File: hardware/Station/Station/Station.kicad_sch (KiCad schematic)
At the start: 7 parts, among them J1 Conn_01x04, J2 Conn_01x04, J3 Conn_01x04, J4 Conn_01x04, J5 Conn_01x04, J6 Conn_01x03

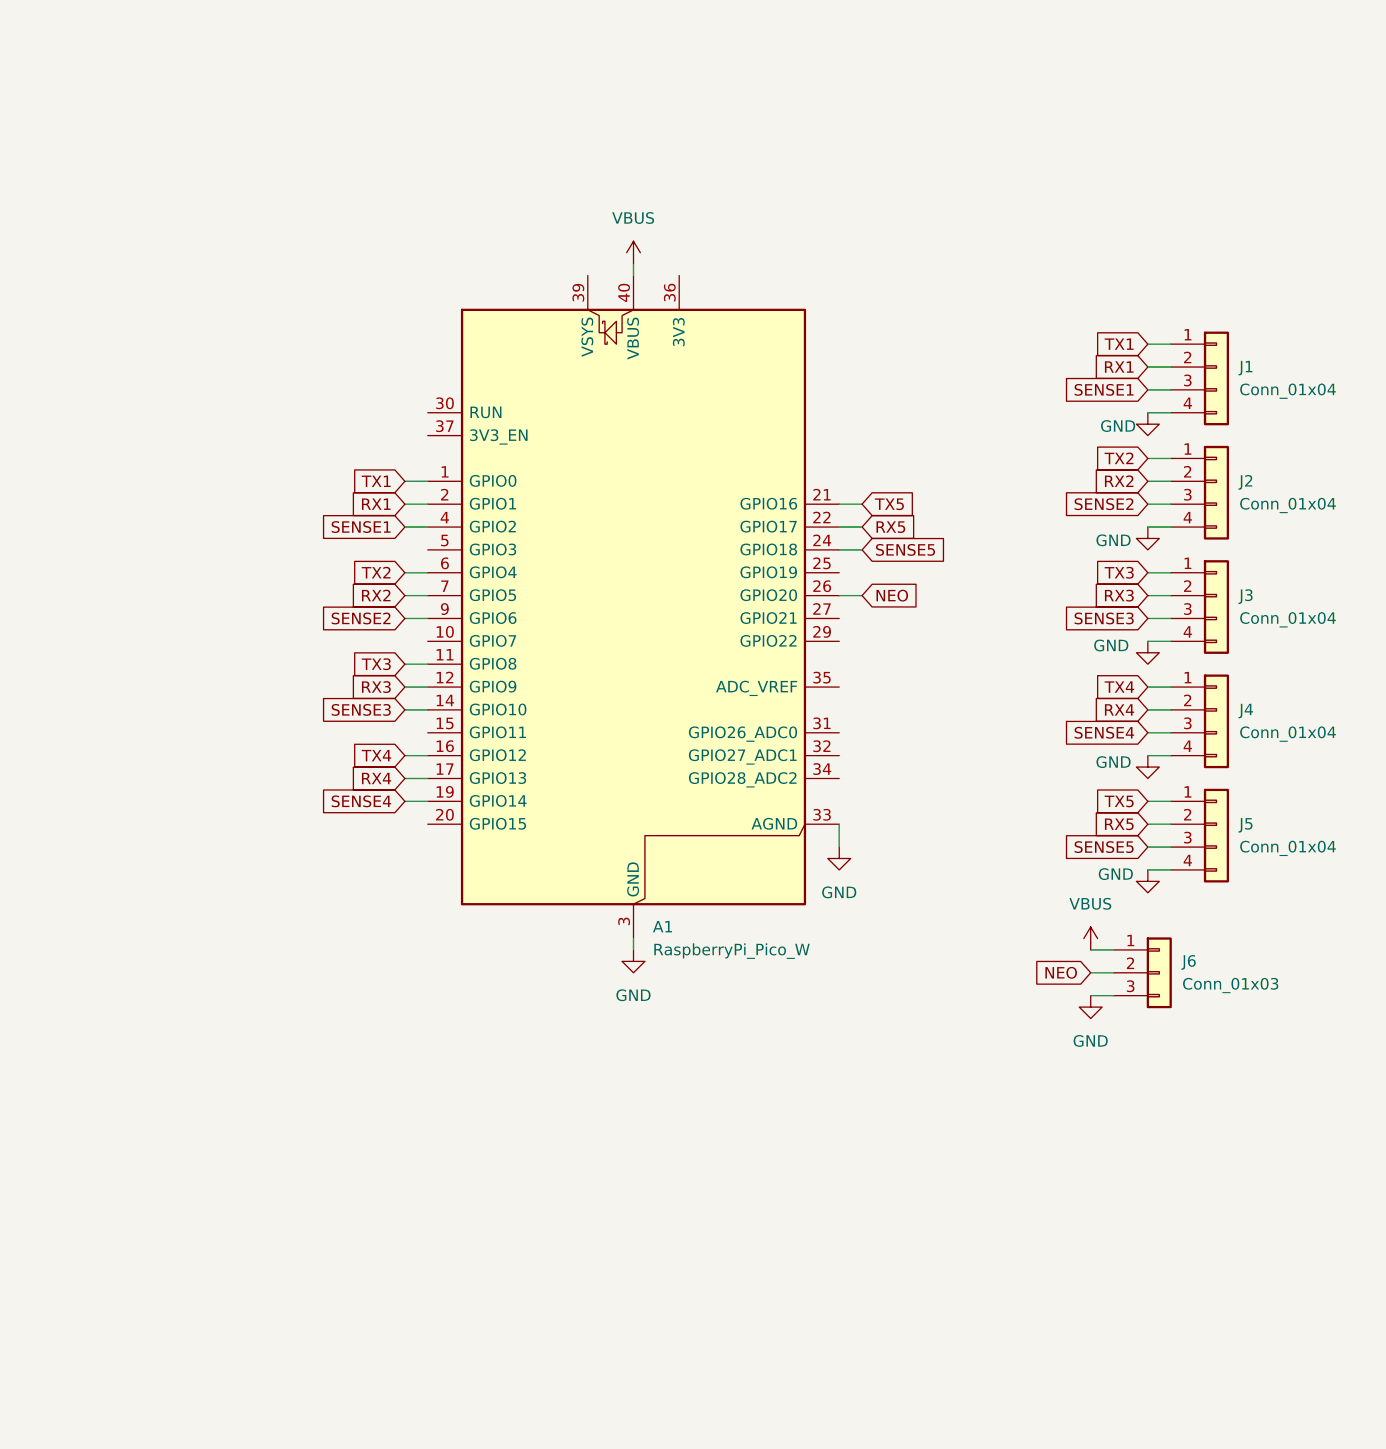
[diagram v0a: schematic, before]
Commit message: V1.0 firmware release
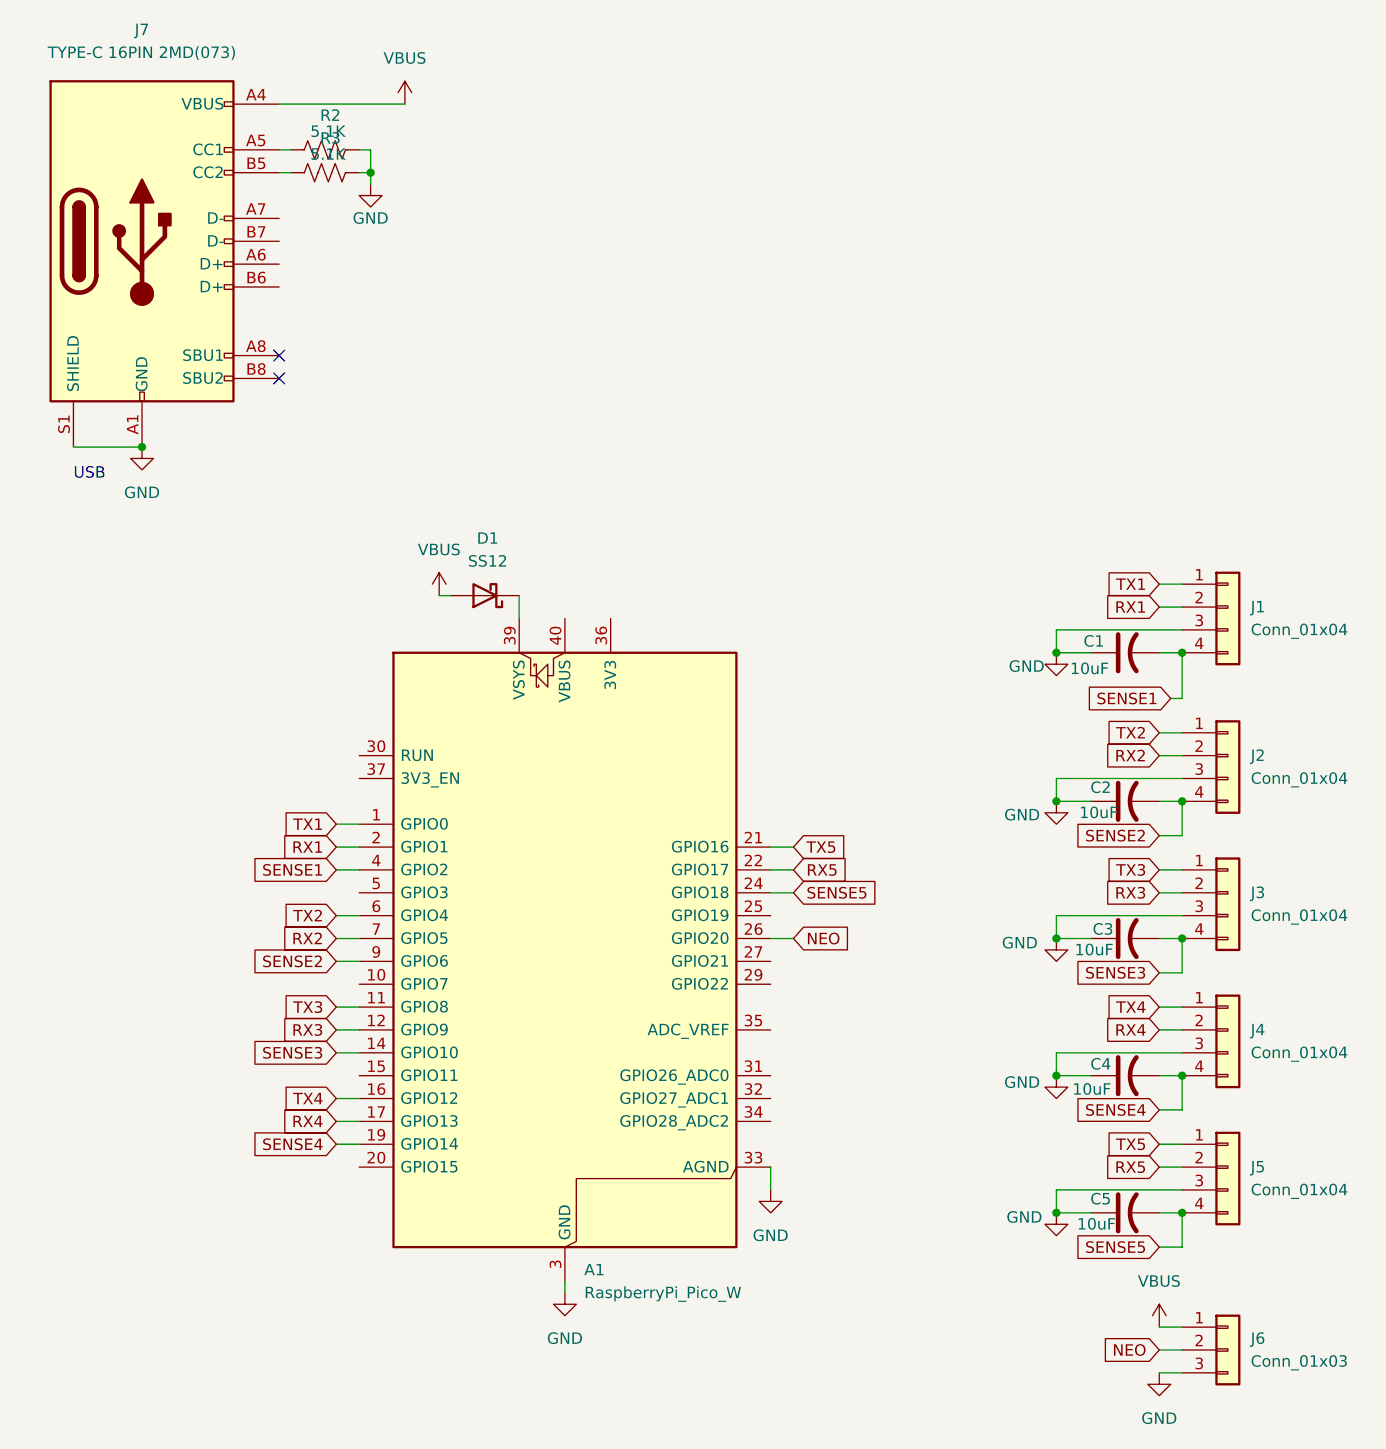
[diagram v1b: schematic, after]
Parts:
- added C1, C2, C3, C4, C5: 10uF, Capacitor_SMD:C_0603_1608Metric_Pad1.08x0.95mm_HandSolder, symbol Device:C_US
- added D1: SS12, Diode_SMD:D_SMA, symbol Diode:SS12
- added J7: TYPE-C 16PIN 2MD(073), Connector_USB:USB_C_Receptacle_GCT_USB4105-xx-A_16P_TopMnt_Horizontal, symbol Connector:USB_C_Receptacle_USB2.0
- added R2, R3: 5.1K, Resistor_SMD:R_0603_1608Metric, symbol Device:R_US
- J1, J2, J3, J4, J5: footprint Connector_PinHeader_1.27mm:PinHeader_1x04_P1.27mm_Vertical -> Connector_PinHeader_2.54mm:PinHeader_1x04_P2.54mm_Vertical
- J6: footprint (none) -> Connector_PinHeader_2.54mm:PinHeader_1x03_P2.54mm_Vertical
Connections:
- net GND: now also J1.3 (Pin_3), J2.3 (Pin_3), J3.3 (Pin_3), J4.3 (Pin_3), J5.3 (Pin_3), C1.1, C2.1, C3.1, C4.1, C5.1, J7.A1 (GND), J7.A12 (GND), J7.B1 (GND), J7.B12 (GND), J7.S1 (SHIELD), R2.2, R3.2; no longer J1.4 (Pin_4), J2.4 (Pin_4), J3.4 (Pin_4), J4.4 (Pin_4), J5.4 (Pin_4)
- net SENSE1: now also J1.4 (Pin_4), C1.2; no longer J1.3 (Pin_3)
- net SENSE2: now also J2.4 (Pin_4), C2.2; no longer J2.3 (Pin_3)
- net SENSE3: now also J3.4 (Pin_4), C3.2; no longer J3.3 (Pin_3)
- net SENSE4: now also J4.4 (Pin_4), C4.2; no longer J4.3 (Pin_3)
- net SENSE5: now also J5.4 (Pin_4), C5.2; no longer J5.3 (Pin_3)
- net VBUS: now also D1.2 (A), J7.A4 (VBUS), J7.A9 (VBUS), J7.B4 (VBUS), J7.B9 (VBUS); no longer A1.40 (VBUS)
- net at A1.39 (VSYS): now also D1.1 (K)
- new net: J7.A5 (CC1), R2.1
- new net: J7.B5 (CC2), R3.1
- no-connect marks 0 -> 2
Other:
- note added: "USB"
- moved on the sheet: A1, J1, J2, J3, J4, J5, J6
